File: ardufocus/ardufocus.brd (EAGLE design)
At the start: 50 x 55 mm, 16 parts, among them J1 PWR, J2 JST, J3 JST, J4 JST, M1 ARDUINO-NANO-3.0

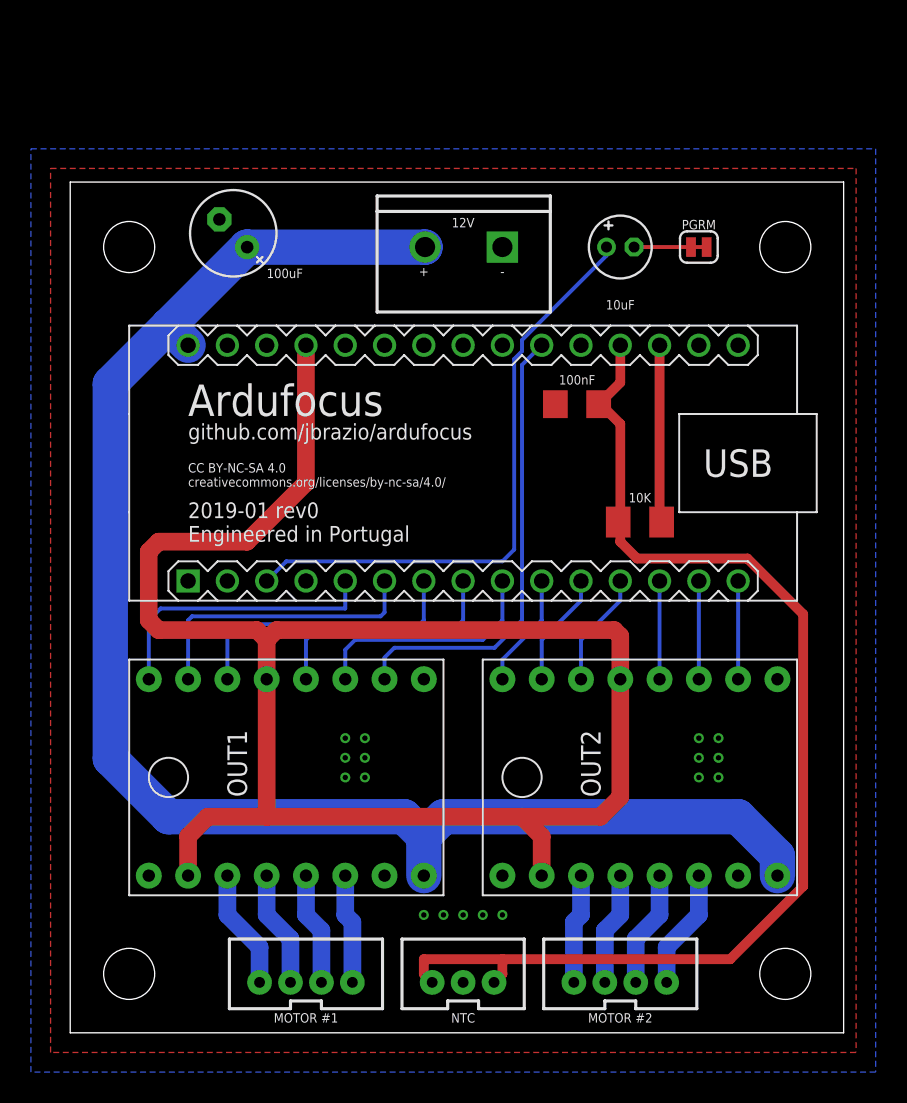
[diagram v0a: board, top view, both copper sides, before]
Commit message: Overall board revision
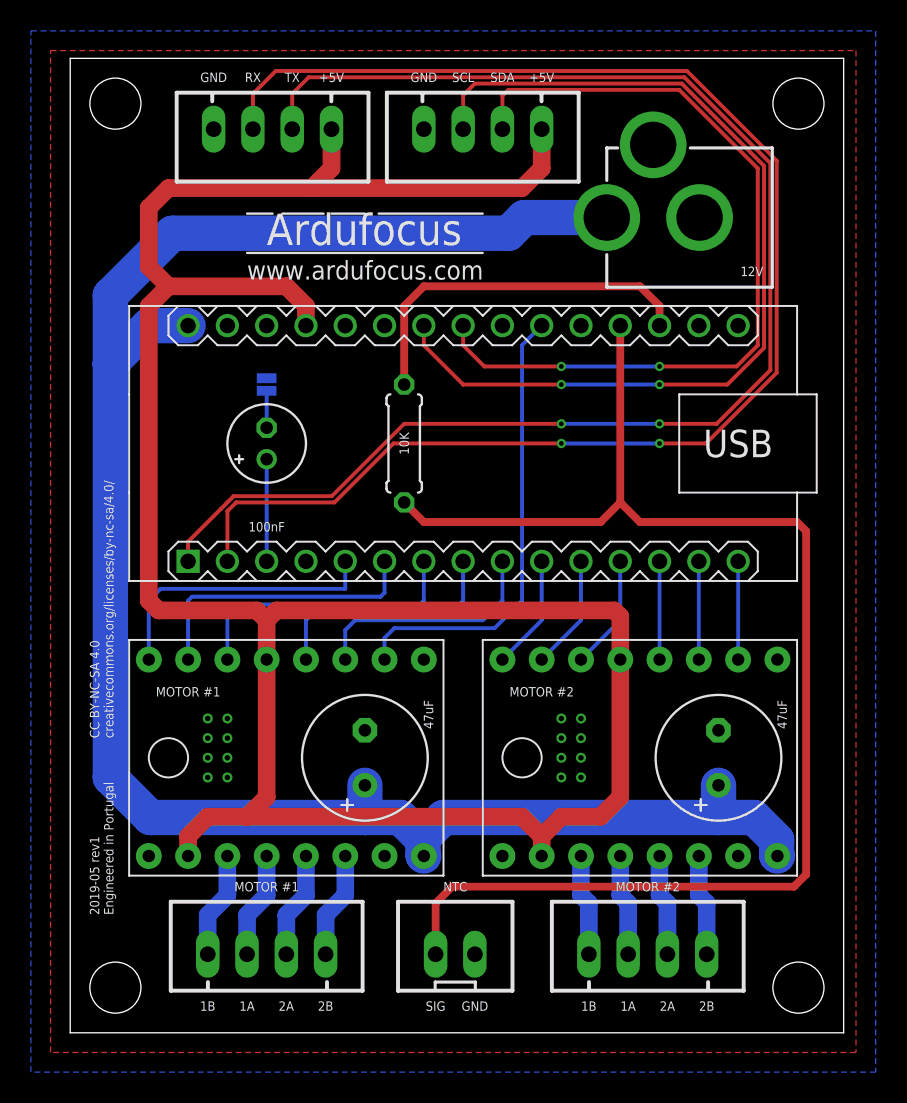
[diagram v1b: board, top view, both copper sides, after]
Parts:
- removed J1: PWR, SparkFun-Connectors:SCREWTERMINAL-5MM-2
- removed J2, J3: JST, SparkFun-Connectors:JST-4-PTH-VERT
- removed J4: JST, SparkFun-Connectors:JST-3-PTH-VERT
- added J5: POWER_JACK, SparkFun-Connectors:POWER_JACK_PTH
- added X2, X3, X4, X5: JST-XH-04-PIN-LONG-PAD, jst-xh:JST-XH-04-PACKAGE-LONG-PAD
- added X6: JST-XH-02-PIN-LONG-PAD, jst-xh:JST-XH-02-PACKAGE-LONG-PAD
- C1: value 10uF -> 100nF; device rcl:E1,8-4 -> rcl:E2-5
- C2: value 10uF -> 47uF; device rcl:E2,5-6E -> rcl:E3,5-8
- C3: value 10nF -> 47uF; device rcl:C3216 -> rcl:E3,5-8
- PGRM: value JUMPER-SMT_2_NC_TRACE_SILK -> JUMPER-SMT_2_NO_SILK; device SparkFun-Jumpers:SMT-JUMPER_2_NC_TRACE_SILK -> SparkFun-Jumpers:SMT-JUMPER_2_NO_SILK
- R1: device rcl:M1206 -> rcl:0207/7
- moved U$3 56.3 mm to (47.1, 60.1)
- moved U$4 47.9 mm to (47.1, 2.92)
- moved C2 35.0 mm to (19.1, 17.8), turned to 90 degrees
- moved PGRM 29.3 mm to (12.7, 41.9), flipped to the bottom, turned to 90 degrees
- moved C1 26.2 mm to (12.7, 38.1), turned to 90 degrees
- moved C3 24.6 mm to (41.9, 17.8), turned to 90 degrees
- moved R1 16.1 mm to (21.6, 38.1), turned to 270 degrees
- moved U$1 9.31 mm to (2.92, 60.1)
- moved M1 1.27 mm to (25.4, 38.1)
- moved OUT1 1.27 mm to (24.1, 10.2)
- moved OUT2 1.27 mm to (47.0, 10.2)
- moved U$2 1.26 mm to (2.92, 2.92)
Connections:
- new net SCL: M1.J2.7, X4.3
- new net SDA: M1.J2.8, X4.2
- net +12V: now also C3.+, J5.PWR; no longer J1.2
- net +5V: now also X4.1, X5.1
- net A0: now also X6.1; no longer C3.1, J4.1, J4.3
- net GND: now also C3.-, J5.GND, X4.4, X5.4, X6.2; no longer C3.2, J1.1, J4.2
- net N$1: now also X3.1; no longer J3.1
- net N$10: now also X3.2; no longer J3.2
- net N$12: now also X3.4; no longer J3.4
- net N$13: now also X2.1; no longer J2.1
- net N$14: now also X2.2; no longer J2.2
- net N$15: now also X2.4; no longer J2.4
- net N$16: now also X3.3; no longer J3.3
- net N$9: now also X2.3; no longer J2.3
- net RX: now also X5.3
- net TX: now also X5.2
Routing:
- net RX: track 0.00 -> 95.3 mm, vias 0 -> 2
- net TX: track 0.00 -> 92.8 mm, vias 0 -> 2
- net SCL: track 0.00 -> 61.2 mm, vias 0 -> 2
- net SDA: track 0.00 -> 53.8 mm, vias 0 -> 2
- net +5V: track 114.5 -> 159.4 mm
- net RST: track 38.9 -> 6.60 mm
- net +12V: track 100.6 -> 123.7 mm
- net A0: track 75.3 -> 89.5 mm
- net AREF: track 11.5 -> 23.9 mm
- net N$2: track 3.68 -> 2.39 mm
- net N$12: track 7.76 -> 6.56 mm
- net N$16: track 7.54 -> 6.56 mm
- net N$13: track 7.76 -> 6.88 mm
- net N$10: track 7.31 -> 6.56 mm
- net N$14: track 7.54 -> 6.88 mm
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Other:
- board size 50 x 55 mm -> 50 x 63 mm
- board text added: "+5V"
- board text added: "1A"
- board text added: "1B"
- board text added: "2019-05 rev1 Engineered in Portugal"
- board text added: "2A"
- board text added: "2B"
- board text added: "47uF"
- board text added: "GND"
- board text added: "RX"
- board text added: "SCL"
- board text added: "SDA"
- board text added: "SIG"
- board text added: "TX"
- board text added: "www.ardufocus.com"
- board text removed: "+"
- board text removed: "-"
- board text removed: "100uF"
- board text removed: "10uF"
- board text removed: "2019-01 rev0 Engineered in Portugal"
- board text removed: "github.com/jbrazio/ardufocus"
